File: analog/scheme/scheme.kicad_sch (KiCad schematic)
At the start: 19 parts, among them U1 Avol=1Meg GBW=10Meg Slew=10Meg, U2 Avol=1Meg GBW=10Meg Slew=10Meg, U3 Avol=1Meg GBW=10Meg Slew=10Meg

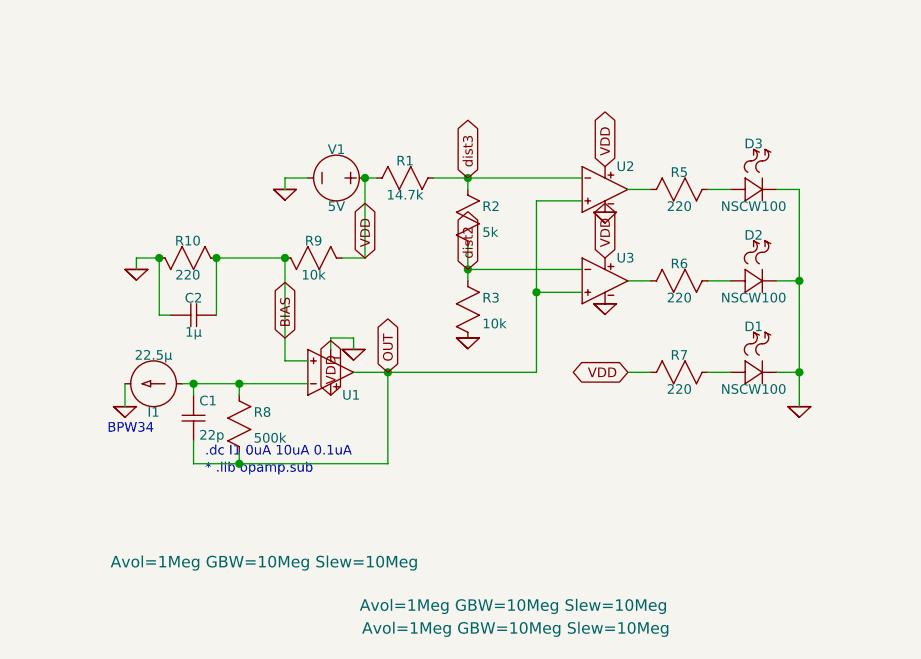
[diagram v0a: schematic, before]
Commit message: better scj´hem
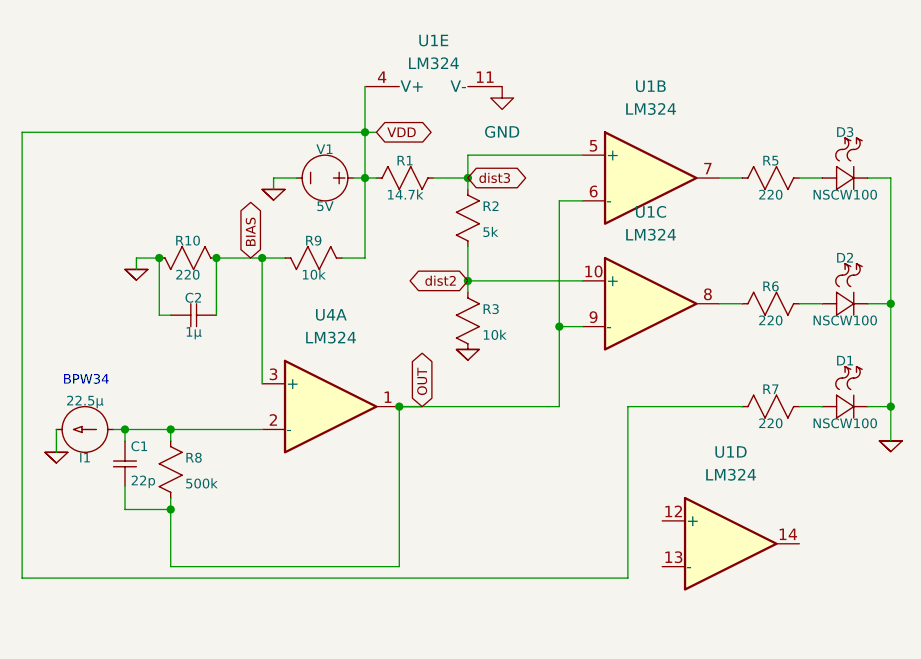
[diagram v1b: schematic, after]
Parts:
- removed U1, U2, U3: Avol=1Meg GBW=10Meg Slew=10Meg, symbol ltspice:OpAmps/UniversalOpAmp2
- added U1, U4: LM324, symbol Amplifier_Operational:LM324
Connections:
- net BIAS: now also U4.3 (+)
- net OUT: now also U1.6 (-), U1.9 (-), U4.1
- net VDD: now also U1.4 (V+)
- net dist2: now also U1.10 (+)
- net dist3: now also U1.5 (+)
- net at C1.1, I1.1 (+), R8.1: now also U4.2 (-)
- net at R6.2: now also U1.8
- net at R5.2: now also U1.7
- new net GND: U1.11 (V-)
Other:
- note removed: "* .lib opamp.sub"
- note removed: ".dc I1 0uA 10uA 0.1uA"
- moved on the sheet: C1, D1, D2, D3, I1, R3, R5, R6, R7, R8, V1

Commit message: n9o cxlue
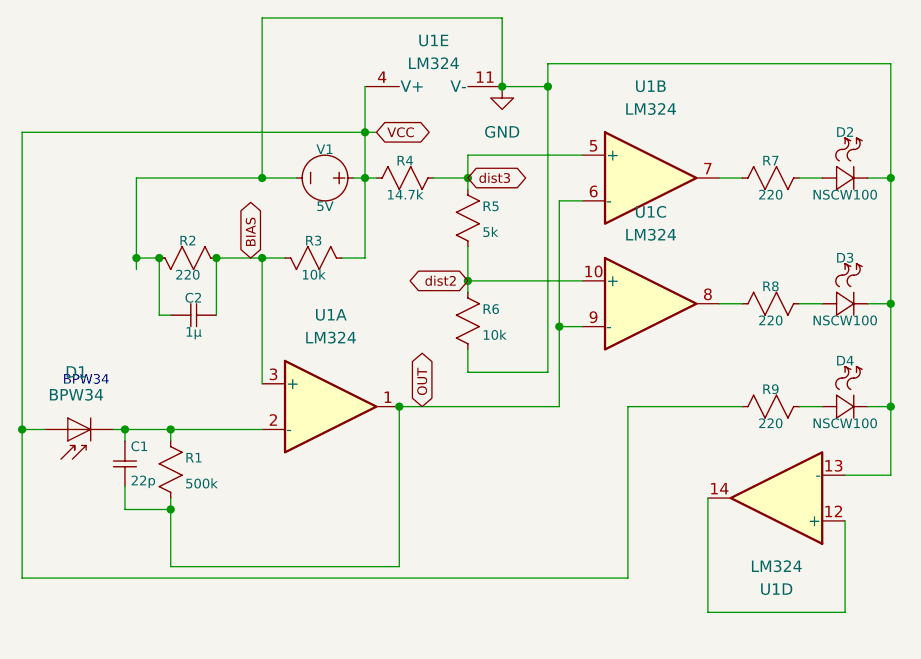
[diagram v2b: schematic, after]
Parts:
- removed I1: 22.5µ, symbol ltspice:current
- removed U4: LM324, symbol Amplifier_Operational:LM324
- added D1: BPW34, OptoDevice:Osram_DIL2_4.3x4.65mm_P5.08mm, symbol Sensor_Optical:BPW34
- added unit 1 of U1
- renumbered D3 to D2, D2 to D3, D1 to D4, R8 to R1, R10 to R2, R9 to R3, R1 to R4, R2 to R5, R3 to R6, R5 to R7, R6 to R8, R7 to R9
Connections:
- net 0 is gone; now on net GND: C2.1, D2.2 (-), D3.2 (-), D4.2 (-), R2.2, R6.2, V1.2 (-)
- net BIAS: now also U1.3 (+)
- net GND: now also U1.13 (-)
- net OUT: now also U1.1
- net at C1.1, R1.1: now also D1.1 (K), U1.2 (-)
- net at U1.12 (+): now also U1.14
- net VDD renamed VCC
- net VCC: now also D1.2 (A)
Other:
- moved on the sheet: U1D
